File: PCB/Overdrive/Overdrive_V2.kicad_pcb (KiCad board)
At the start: 2 copper layers, 89 x 76.3 mm, 47 parts, among them J1 Alimentación, J2 Entrada, J3 Salida, J4 LM1117_3.3V, SW2 BT_sw, U1 TL072, U2 TL072

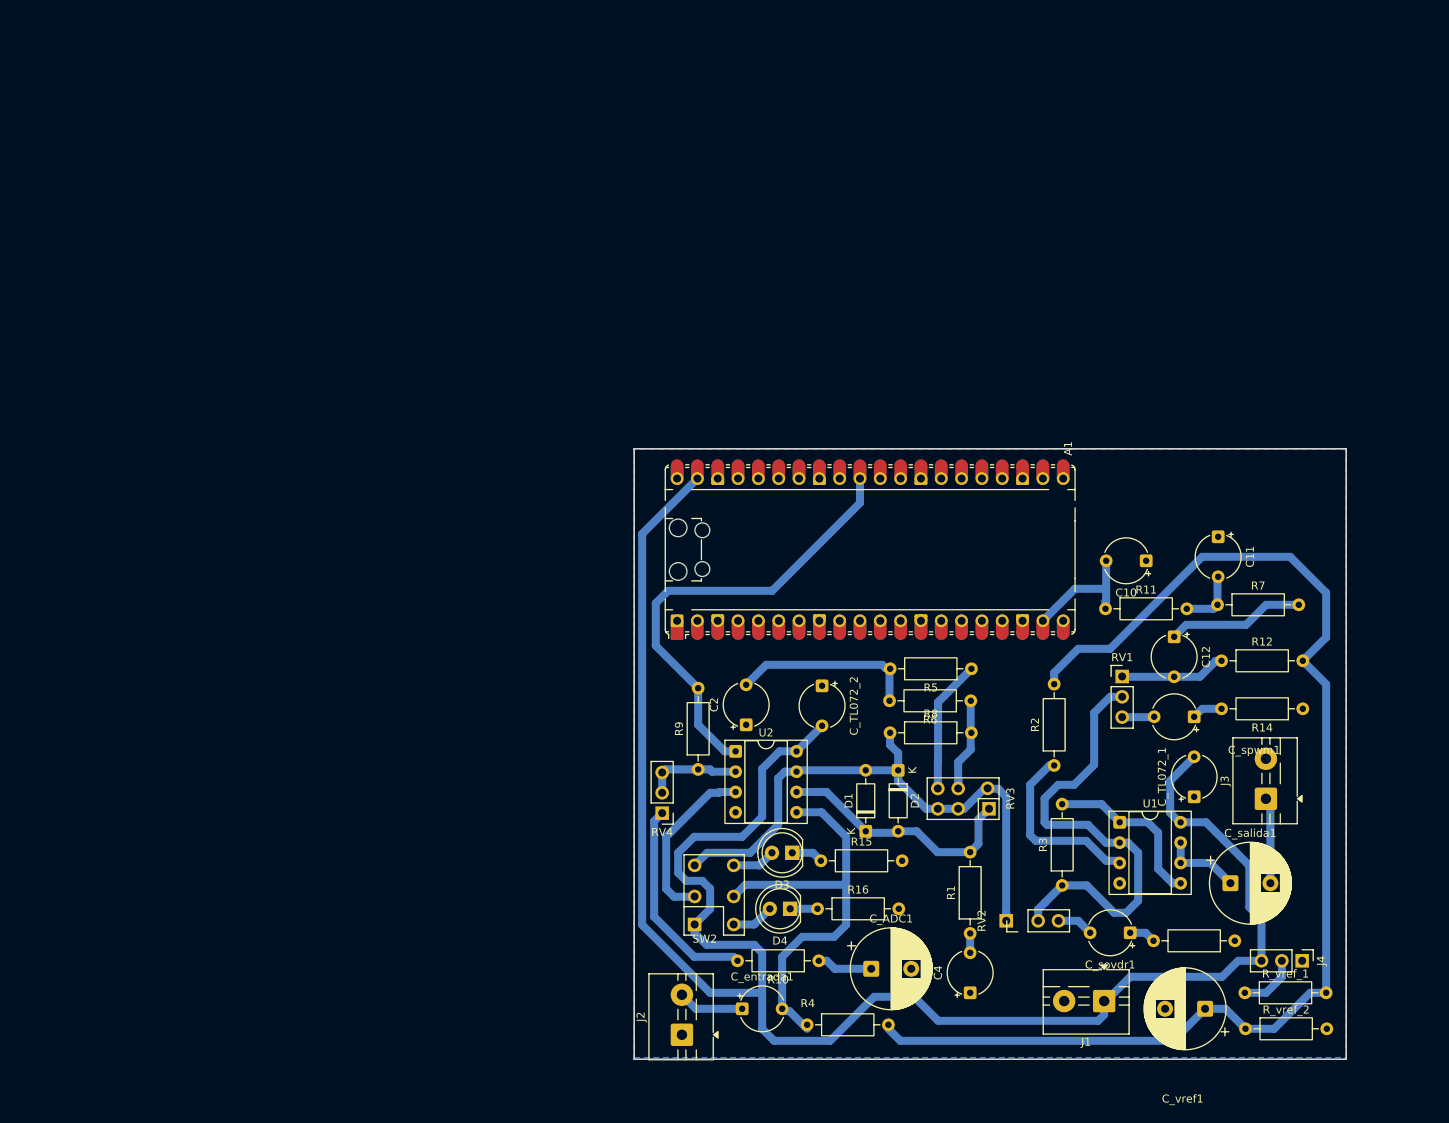
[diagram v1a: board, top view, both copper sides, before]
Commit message: A
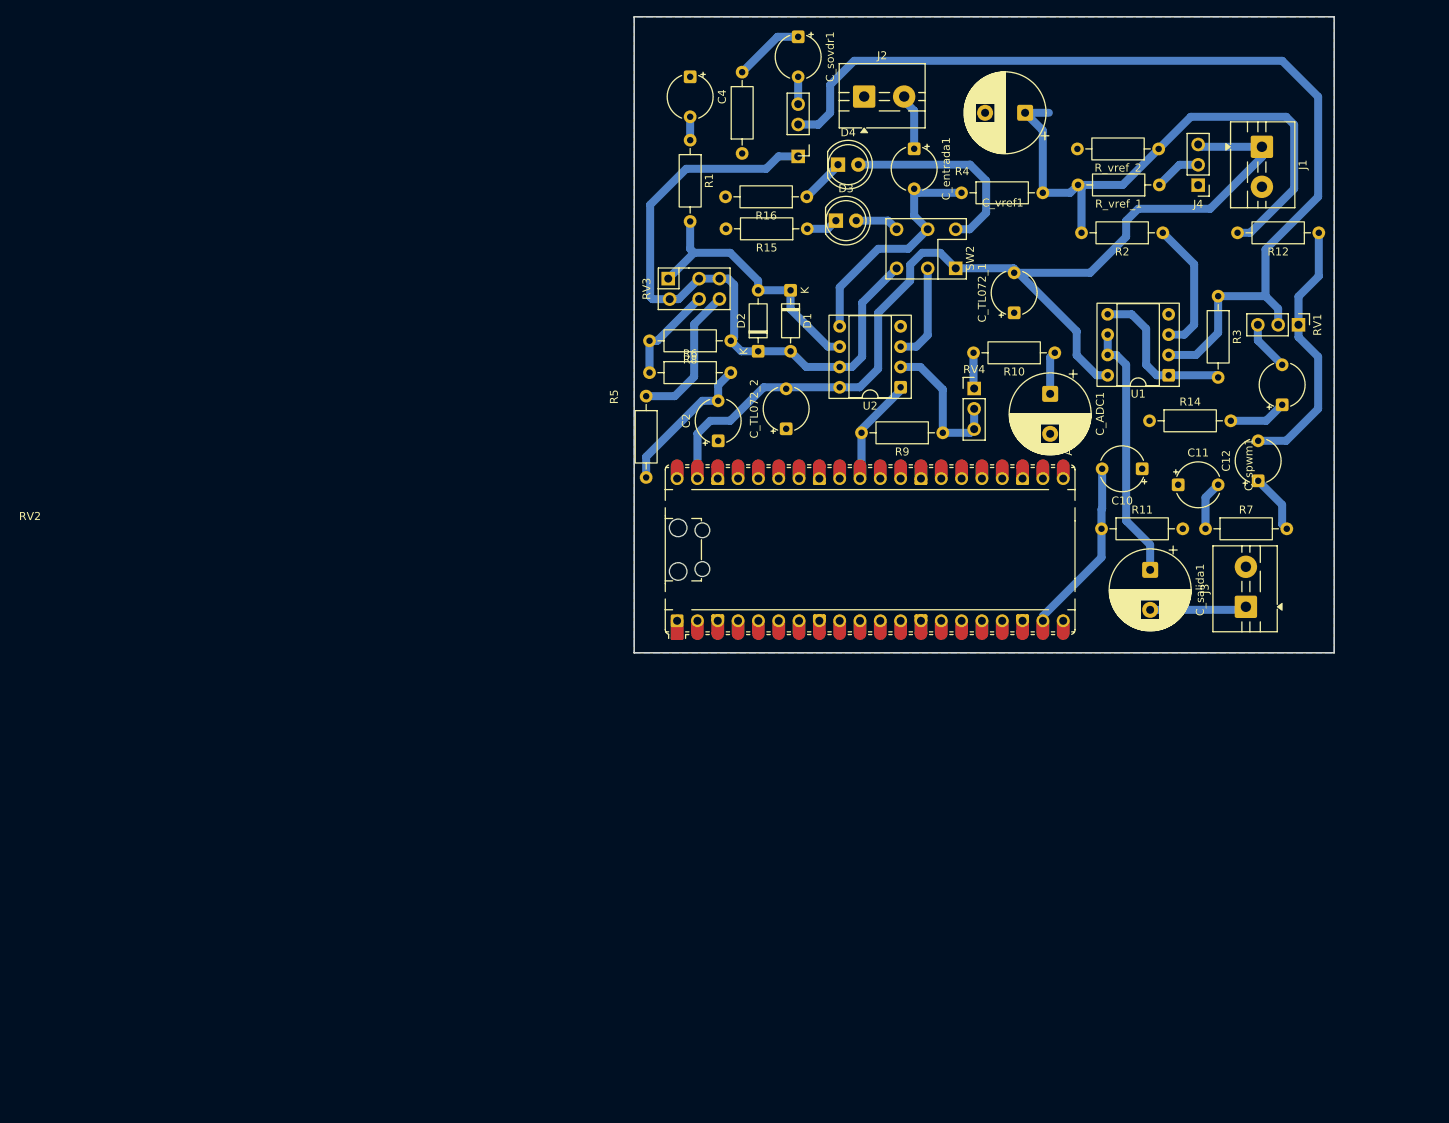
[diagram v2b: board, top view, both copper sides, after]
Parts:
- moved C4 119.7 mm to (37.5, 75.0), turned to -90 degrees
- moved J2 119.5 mm to (59.2, 77.5), turned to 0 degrees
- moved C_sovdr1 119.4 mm to (51.0, 70.0), turned to -90 degrees
- moved R13 116.1 mm to (44.0, 84.6), turned to 90 degrees
- moved C_vref1 114.2 mm to (79.4, 79.5)
- moved R_vref_2 110.5 mm to (96.1, 84.0), turned to 180 degrees
- moved C_entrada1 109.6 mm to (65.5, 84.0), turned to -90 degrees
- moved J1 108.6 mm to (109.0, 83.8), turned to -90 degrees
- moved R4 105.8 mm to (71.4, 89.5)
- moved R1 105.2 mm to (37.5, 82.9), turned to -90 degrees
- moved R_vref_1 101.5 mm to (96.1, 88.5), turned to 180 degrees
- moved RV2 100.8 mm to (51.0, 83.5), turned to 180 degrees
- moved J4 97.8 mm to (101.0, 88.5), turned to 180 degrees
- moved D4 93.2 mm to (56.0, 86.0), turned to 0 degrees
- moved R16 89.0 mm to (52.1, 90.0), turned to 180 degrees
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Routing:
- net Vcc: track 241.9 -> 127.1 mm
- net Vref: track 155.6 -> 73.2 mm
- net Net-(U1A--): track 58.2 -> 122.0 mm
- net ADC_IN: track 57.2 -> 13.5 mm
- net Net-(SW2A-A): track 53.4 -> 30.8 mm
- net Net-(U1B--): track 9.81 -> 32.2 mm
- net Net-(R10-Pad2): track 26.1 -> 4.49 mm
- net Net-(D4-A): track 5.33 -> 25.5 mm
- net Net-(C12-Pad2): track 13.3 -> 33.2 mm
- net Net-(D1-A): track 72.1 -> 82.8 mm
- net Net-(C12-Pad1): track 17.2 -> 7.48 mm
- net Net-(SW2A-B): track 21.5 -> 12.3 mm
- net Net-(U2A--): track 12.0 -> 18.5 mm
- net PWM_out: track 15.6 -> 22.1 mm
- net Net-(U1A-+): track 22.9 -> 16.8 mm
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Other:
- board size 89 x 76.3 mm -> 87.5 x 79.5 mm

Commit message: A
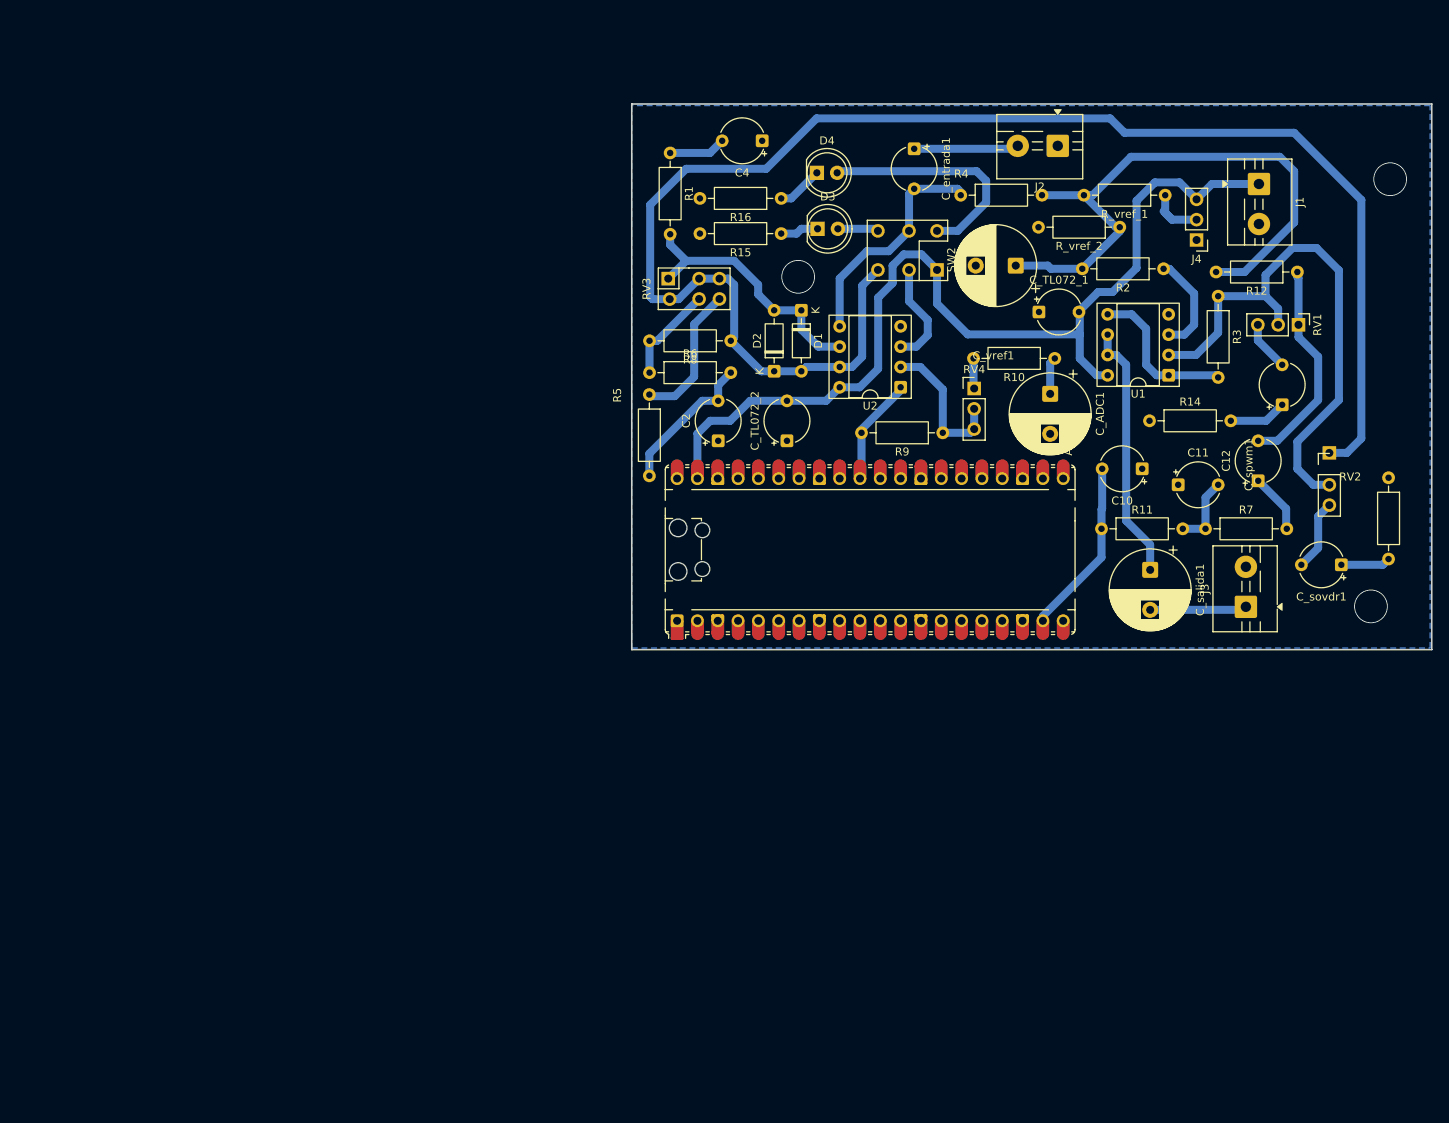
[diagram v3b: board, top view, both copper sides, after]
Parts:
- moved C_sovdr1 94.7 mm to (118.9, 136.0), turned to 180 degrees
- moved R13 90.4 mm to (124.8, 125.1), turned to -90 degrees
- moved RV2 77.5 mm to (117.4, 123.5), turned to 0 degrees
- moved J2 25.0 mm to (83.5, 83.6), turned to 180 degrees
- moved C_vref1 19.1 mm to (78.2, 98.6)
- moved C4 12.0 mm to (46.5, 83.0), turned to 180 degrees
- moved R_vref_2 10.9 mm to (91.2, 93.8)
- moved J4 6.86 mm to (100.8, 95.4)
- moved R12 5.59 mm to (113.4, 99.4)
- moved J1 4.66 mm to (108.6, 88.4)
- moved R2 4.50 mm to (96.7, 99.0)
- moved R15 3.31 mm to (48.9, 94.6)
- moved R16 3.21 mm to (48.9, 90.2)
- moved D2 3.20 mm to (48.0, 111.8)
- moved C_TL072_1 3.10 mm to (81.1, 104.4), turned to 0 degrees
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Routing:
- net Net-(D1-A): track 82.8 -> 193.2 mm
- net Net-(U1A--): track 122.0 -> 68.2 mm
- net Net-(C12-Pad2): track 33.2 -> 26.7 mm
- net Net-(J2-Pin_2): track 7.05 -> 13.1 mm
- net Net-(C_sovdr1-Pad2): track 3.42 -> 8.91 mm
- net Vcc: track 127.1 -> 121.7 mm
- net Net-(C4-Pad2): track 2.92 -> 7.13 mm
- net Net-(U1A-+): track 16.8 -> 12.7 mm
- net Net-(D4-A): track 25.5 -> 29.5 mm
- net Net-(C11-Pad2): track 6.15 -> 8.99 mm
- net Net-(C_sovdr1-Pad1): track 8.83 -> 6.20 mm
- net 3.3V: track 5.90 -> 7.98 mm
- net Net-(SW2A-A): track 30.8 -> 28.8 mm
- net Vref: track 73.2 -> 74.7 mm
- net Net-(D3-K): track 4.00 -> 4.80 mm
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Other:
- board size 87.5 x 79.5 mm -> 100 x 68.2 mm
